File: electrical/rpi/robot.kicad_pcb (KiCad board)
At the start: 2 copper layers, 42.5 x 15.2 mm, 9 parts, among them J1 i2c, J2 Pi Header, J4 i2c, J6 Power/Data Input, Q1 BSS138, U2 74-125, U3 74-126

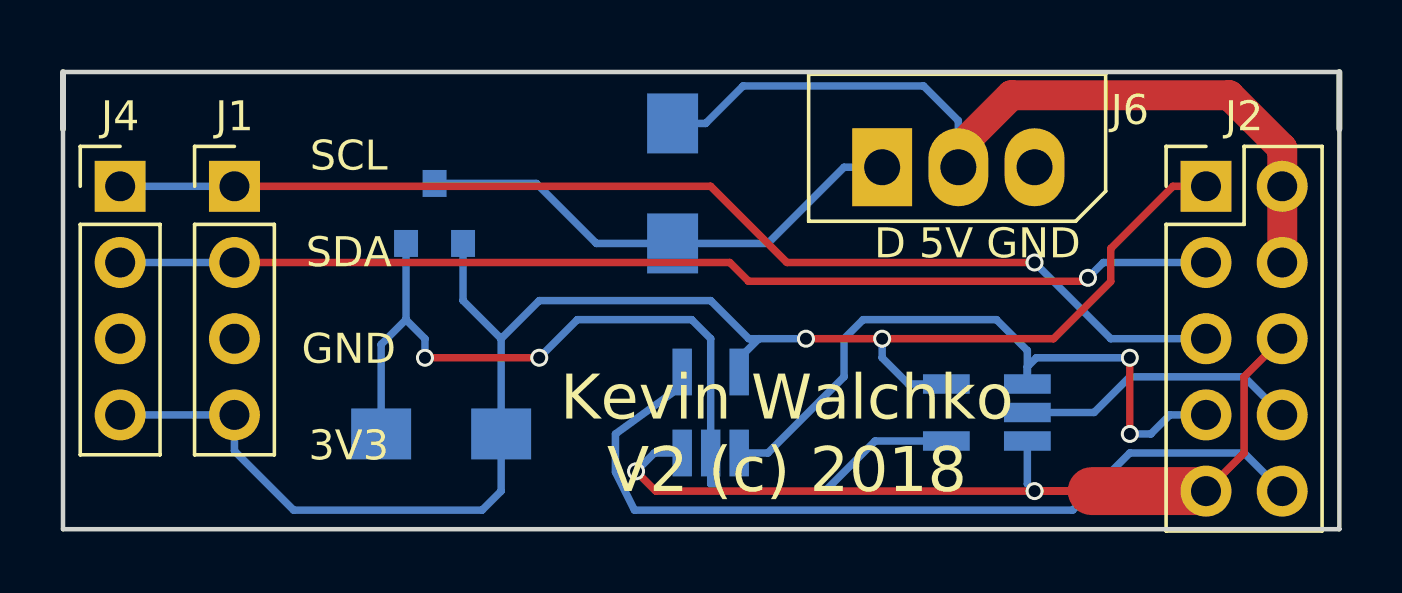
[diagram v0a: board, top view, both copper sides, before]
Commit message: new board :electric_plug:  :bento:
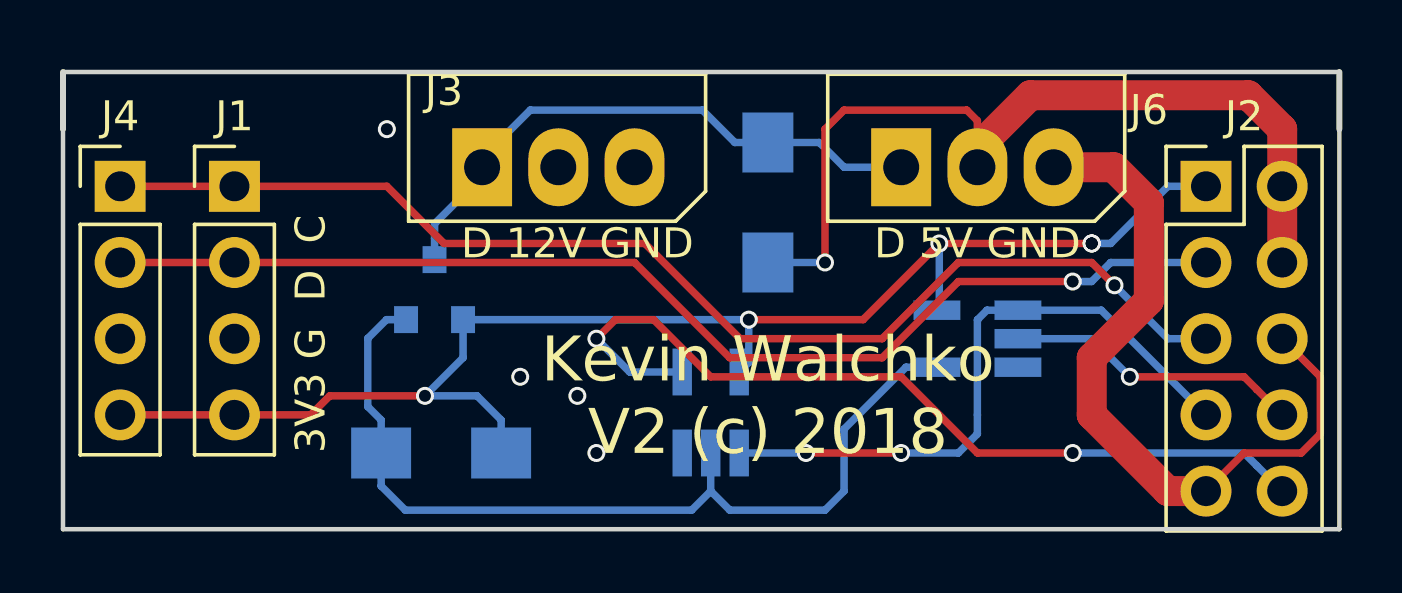
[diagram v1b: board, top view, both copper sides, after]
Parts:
- added J3: 12V/Data, Connectors_Molex:Molex_SPOX-5267_22-03-5035_03x2.54mm_Straight, F.Cu at (146.1, 59.1)
- J6: value Power/Data Input -> 5V/Data
- U2: value 74-125 -> 74L-125
- U3: value 74-126 -> 74L-126
- moved R2 3.24 mm to (155.6, 60.2), turned to 90 degrees
- moved Q1 2.54 mm to (144.5, 63.1)
- moved U3 2.48 mm to (162.6, 64.8)
- moved J6 0.64 mm to (160.0, 59.1)
- moved R3 0.64 mm to (144.7, 68.6)
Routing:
- net +3V3: track 55.6 -> 48.2 mm, vias 2 -> 5
- net GND: track 30.9 -> 24.7 mm, vias 2 -> 4
- net DATA: track 16.8 -> 19.5 mm
- net +5V: track 28.8 -> 31.1 mm, vias 0 -> 1
- net SDA: track 36.7 -> 38.8 mm
- net SCL: track 38.3 -> 40.4 mm
- net DTR: track 23.2 -> 21.2 mm
- net Net-(Q1-Pad2): track 32.0 -> 30.5 mm, vias 2 -> 0
- net TXO: track 9.51 -> 9.86 mm, vias 0 -> 1
- net RXI: vias 0 -> 2
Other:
- board text added: "3V3 G D C"
- board text added: "D 12V GND"
- board text removed: "SCL SDA GND 3V3"
